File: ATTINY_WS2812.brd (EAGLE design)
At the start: 58.4 x 55.9 mm, 36 parts, among them J1 POWER_JACKPTH, U2 ATTINY2313A, Y1 16MHZ

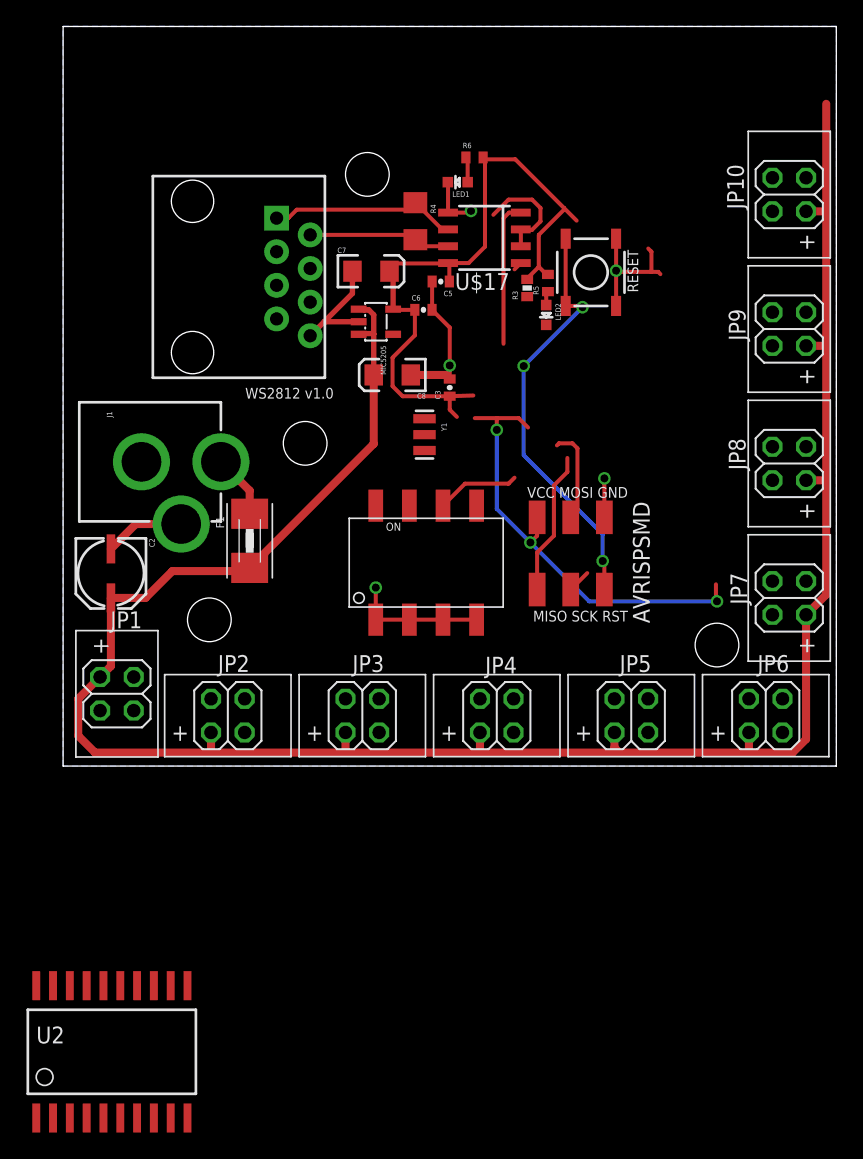
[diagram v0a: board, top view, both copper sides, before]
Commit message: attiny2313 control board
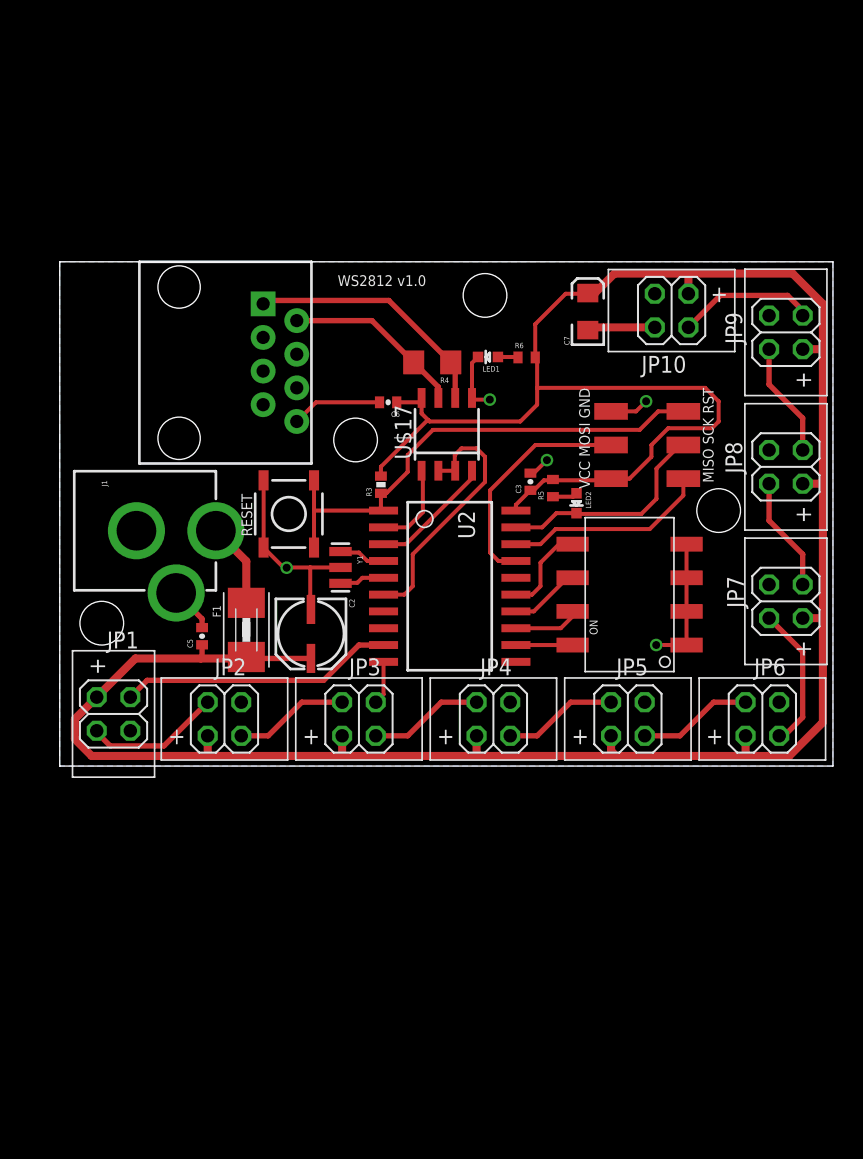
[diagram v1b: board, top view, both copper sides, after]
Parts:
- removed C8: 10uF, SparkFun:EIA3216
- removed MIC5205: ###V, SparkFun:SOT23-5
- moved STANDOFF2 46.5 mm to (3.17, 10.8)
- moved U2 43.5 mm to (29.5, 13.6), turned to 270 degrees
- moved STANDOFF3 39.4 mm to (49.8, 19.3)
- moved C5 32.3 mm to (10.8, 9.81), turned to 90 degrees
- moved RESET 29.2 mm to (17.3, 19.0), turned to 90 degrees
- moved R3 18.5 mm to (24.3, 21.3)
- moved C7 16.7 mm to (39.9, 34.3), turned to 90 degrees
- moved C2 15.8 mm to (19.2, 10.0)
- moved R6 15.6 mm to (35.3, 30.9)
- moved U$21 15.6 mm to (43.1, 13.0), turned to 90 degrees
- moved R5 15.5 mm to (37.3, 21.0)
- moved U$17 15.1 mm to (29.2, 25.1), turned to 0 degrees
- moved LED2 14.4 mm to (39.0, 19.9)
- moved LED1 13.4 mm to (32.4, 30.9)
- moved STANDOFF1 12.8 mm to (32.1, 35.6)
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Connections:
- removed net DI: JP1.3
- removed net N$5: U$21.1, U$21.2, U$21.3, U$21.4
- removed net PB0: U$21.5, U2.12
- removed net PB1: U$21.6, U2.13
- removed net PB2: U$21.7, U2.14
- removed net PB3: U$21.8, U2.15
- removed net VDD: C2.+, C8.A, F1.2, JP1.4, JP10.4, JP2.4, JP3.4, JP4.4, JP5.4, JP6.4, JP7.4, JP8.4, JP9.4, MIC5205.1, MIC5205.3
- new net N$1: U$21.5, U2.15
- new net N$3: U$21.6, U2.14
- new net N$6: U$21.7, U2.13
- new net N$9: U$21.8, U2.12
- net GND: now also U$21.1, U$21.2, U$21.3, U$21.4; no longer C8.C, MIC5205.2
- net VCC: now also C2.+, F1.2, JP1.4, JP10.4, JP2.4, JP3.4, JP4.4, JP5.4, JP6.4, JP7.4, JP8.4, JP9.4; no longer MIC5205.5
- net WS: now also JP1.3
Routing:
- net VDD: track 165.5 -> 0.00 mm
- net VCC: track 86.0 -> 211.2 mm, vias 3 -> 0
- net WS: track 0.00 -> 20.8 mm
- net SCK: track 1.76 -> 16.6 mm
- net RE/DE: track 8.35 -> 19.7 mm
- net DO-6: track 0.00 -> 10.9 mm
- net DO-9: track 0.00 -> 10.5 mm
- net DO-1: track 0.00 -> 10.3 mm
- net MOSI: track 7.20 -> 17.5 mm
- net N$5: track 10.0 -> 0.00 mm, vias 1 -> 0
- net GND: track 43.9 -> 53.4 mm, vias 4 -> 5
- net DO-5: track 0.00 -> 8.67 mm
- net DO-2: track 0.00 -> 8.67 mm
- net DO-8: track 0.00 -> 8.67 mm
- net DO-7: track 0.00 -> 8.67 mm
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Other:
- board size 58.4 x 55.9 mm -> 58.4 x 38.1 mm
